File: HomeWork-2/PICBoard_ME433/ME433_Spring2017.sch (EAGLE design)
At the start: 13 parts, among them J6 USB_MINI-B_SMT, Q1 MCP1702

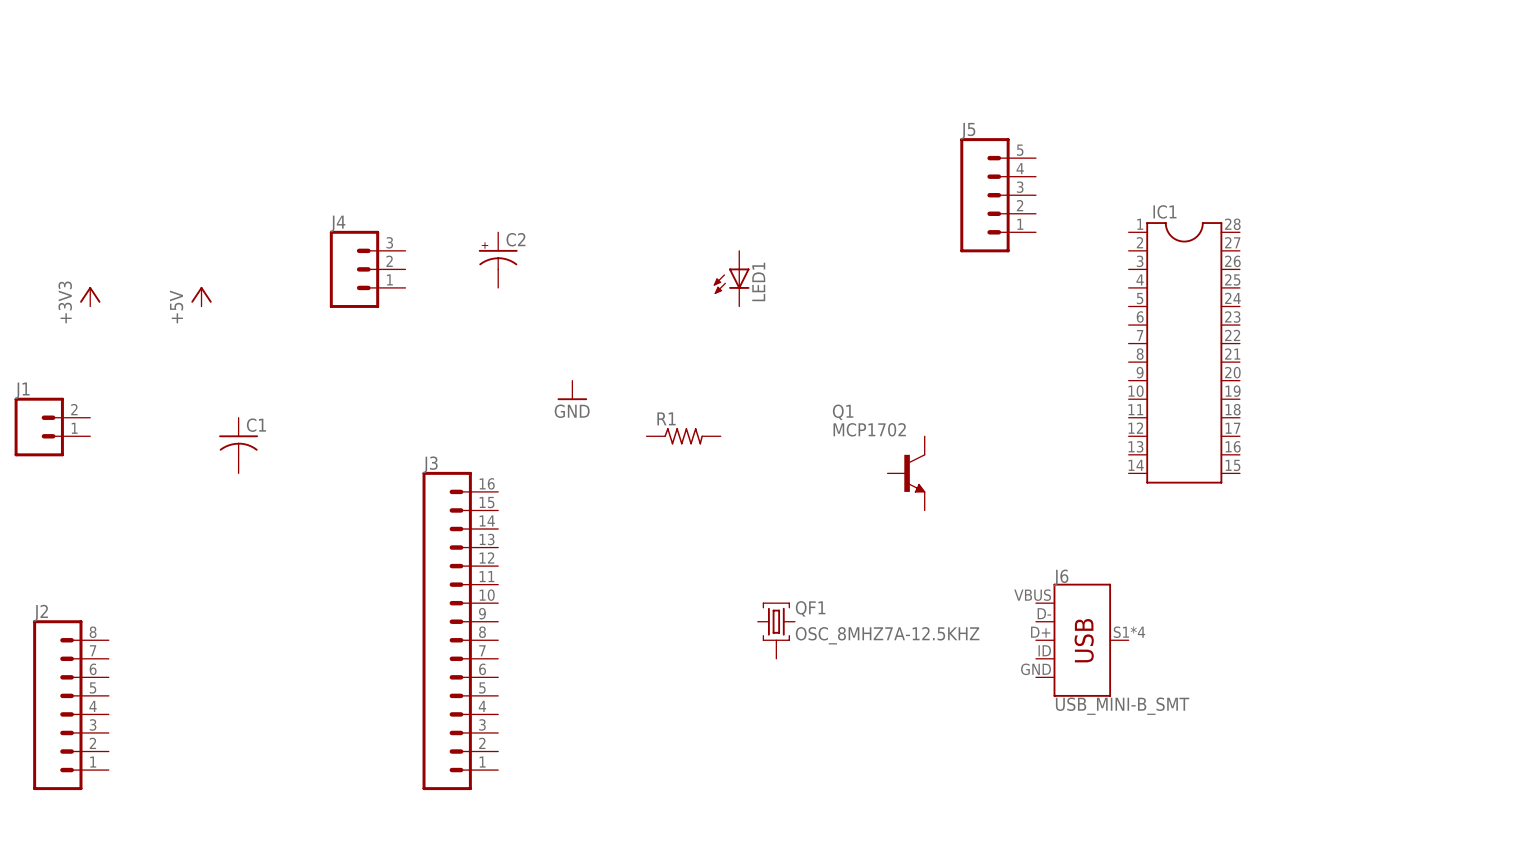
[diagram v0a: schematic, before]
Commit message: Schematic Version #1
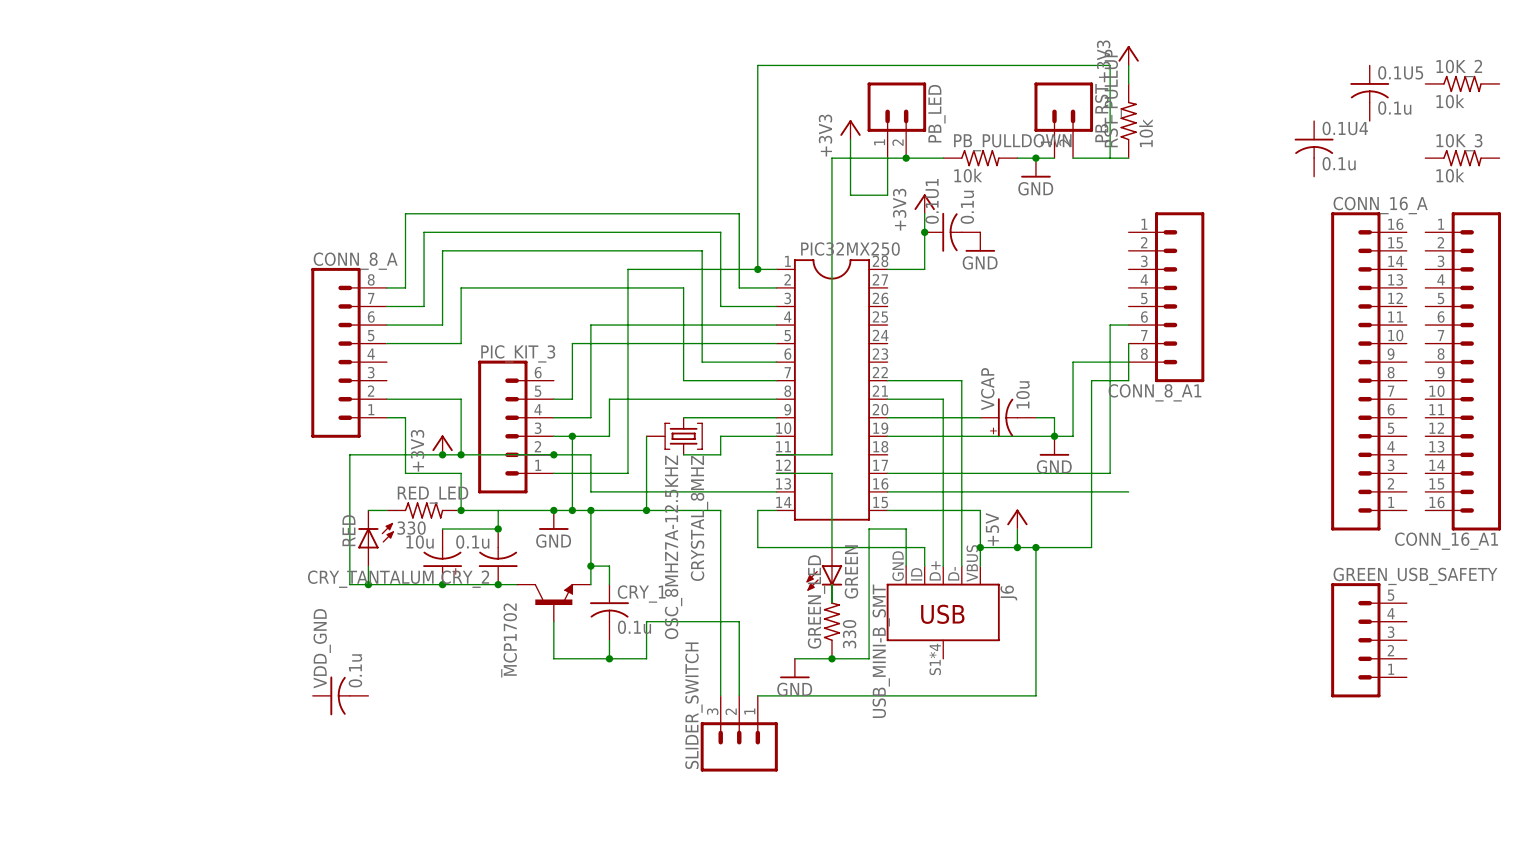
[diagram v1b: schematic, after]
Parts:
- removed C1: (no value), ME433_Spring2017:C-US025-025X050
- removed C2: (no value), ME433_Spring2017:CPOL-USB45181B
- removed IC1: (no value), ME433_Spring2017:PIC-3
- removed J1: (no value), ME433_Spring2017:BUTTONS
- removed J2: (no value), ME433_Spring2017:CONN_08"
- removed J3: (no value), ME433_Spring2017:CONN_16
- removed J4: (no value), ME433_Spring2017:SLIDER_SWITCH
- removed J5: (no value), ME433_Spring2017:USB_GREENBOARD_PULLOUT
- removed LED1: (no value), ME433_Spring2017:LEDSFH482
- removed Q1: MCP1702, ME433_Spring2017:MCP1702
- removed QF1: OSC_8MHZ7A-12.5KHZ, ME433_Spring2017:OSC_8MHZ7A-12.5KHZ
- removed R1: (no value), ME433_Spring2017:R-US_0204/7
- added 0.1U1, 0.1U4, 0.1U5, CRY_1, CRY_2, VDD_GND: 0.1u, ME433_Spring2017:C-US025-025X050
- added 10K_2, 10K_3, PB_PULLDOWN, RST_PULLUP: 10k, ME433_Spring2017:R-US_0204/7
- added CONN_16_A, CONN_16_A1: (no value), ME433_Spring2017:CONN_16
- added CONN_8_A, CONN_8_A1: (no value), ME433_Spring2017:CONN_08"
- added CRYSTAL_8MHZ: OSC_8MHZ7A-12.5KHZ, ME433_Spring2017:OSC_8MHZ7A-12.5KHZ
- added CRY_TANTALUM, VCAP: 10u, ME433_Spring2017:CPOL-USB45181B
- added GREEN, RED: (no value), ME433_Spring2017:LEDSFH482
- added GREEN_LED, RED_LED: 330, ME433_Spring2017:R-US_0204/7
- added GREEN_USB_SAFETY: (no value), ME433_Spring2017:USB_GREENBOARD_PULLOUT
- added PB_LED, PB_RST: (no value), ME433_Spring2017:BUTTONS
- added PIC32MX250: (no value), ME433_Spring2017:PIC-3
- added PIC_KIT_3: (no value), ME433_Spring2017:PICKIT3NO_SILK_FEMALE_PTH
- added SLIDER_SWITCH: (no value), ME433_Spring2017:SLIDER_SWITCH
- added _: MCP1702, ME433_Spring2017:MCP1702
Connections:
- new net +3V3: 0.1U1.1, CONN_8_A.2, CRY_2.1, CRY_TANTALUM.+, PB_LED.1, PIC32MX250.13, PIC32MX250.28, PIC_KIT_3.2, RED.A, RST_PULLUP.2, _.C
- new net +5V: CONN_8_A1.7, J6.VBUS, PIC32MX250.15, SLIDER_SWITCH.1
- new net GND: 0.1U1.2, CONN_8_A.1, CONN_8_A1.8, CRYSTAL_8MHZ.2, CRY_1.1, CRY_2.2, CRY_TANTALUM.-, GREEN_LED.1, J6.GND, PB_PULLDOWN.2, PB_RST.1, PIC32MX250.19, PIC32MX250.8, PIC_KIT_3.3, RED_LED.2, SLIDER_SWITCH.3, VCAP.-, _.E
- new net N$1: CONN_8_A.8, PIC32MX250.2
- new net N$10: PB_LED.2, PB_PULLDOWN.1, PIC32MX250.11
- new net N$11: PIC32MX250.20, VCAP.+
- new net N$12: J6.D+, PIC32MX250.21
- new net N$13: J6.D-, PIC32MX250.22
- new net N$14: CRY_1.2, SLIDER_SWITCH.2, _.B
- new net N$15: PB_RST.2, PIC32MX250.1, PIC_KIT_3.1, RST_PULLUP.1
- new net N$16: RED.C, RED_LED.1
- new net N$17: CONN_8_A.7, PIC32MX250.3
- new net N$18: CONN_8_A.5, PIC32MX250.7
- new net N$2: PIC32MX250.4, PIC_KIT_3.4
- new net N$22: PIC32MX250.16
- new net N$23: CONN_8_A1.6, PIC32MX250.17
- new net N$3: PIC32MX250.5, PIC_KIT_3.5
- new net N$4: GREEN.A, PIC32MX250.12
- new net N$5: CRYSTAL_8MHZ.1, PIC32MX250.9
- new net N$6: CRYSTAL_8MHZ.3, PIC32MX250.10
- new net N$7: GREEN.C, GREEN_LED.2
- new net N$8: J6.ID, PIC32MX250.14
- new net N$9: CONN_8_A.6, PIC32MX250.6
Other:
- moved on the sheet: J6

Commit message: Schematic Version #2
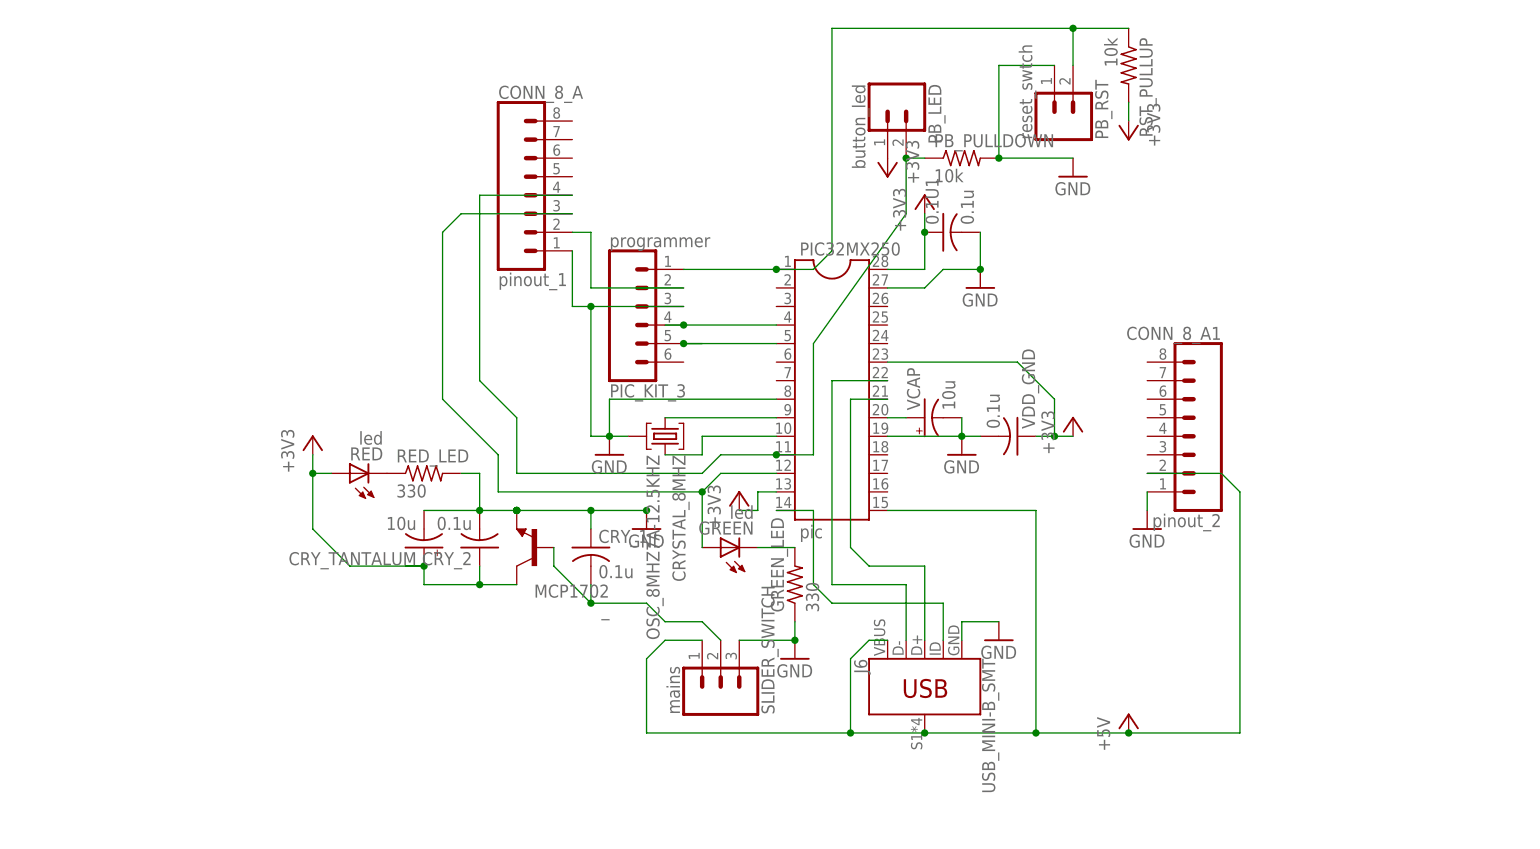
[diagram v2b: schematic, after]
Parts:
- removed 0.1U4, 0.1U5: 0.1u, ME433_Spring2017:C-US025-025X050
- removed 10K_2, 10K_3: 10k, ME433_Spring2017:R-US_0204/7
- removed CONN_16_A, CONN_16_A1: (no value), ME433_Spring2017:CONN_16
- removed GREEN_USB_SAFETY: (no value), ME433_Spring2017:USB_GREENBOARD_PULLOUT
- CONN_8_A: value (none) -> pinout_1
- CONN_8_A1: value (none) -> pinout_2
- GREEN, RED: value (none) -> led
- PB_LED: value (none) -> button_led
- PB_RST: value (none) -> reset_swtch
- PIC32MX250: value (none) -> pic
- PIC_KIT_3: value (none) -> programmer
- SLIDER_SWITCH: value (none) -> mains
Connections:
- removed net N$17: CONN_8_A.7, PIC32MX250.3
- removed net N$18 (its old number): CONN_8_A.5, PIC32MX250.7
- removed net N$22: PIC32MX250.16
- removed net N$23: CONN_8_A1.6, PIC32MX250.17
- removed net N$4 (its old number): GREEN.A, PIC32MX250.12
- removed net N$9 (its old number): CONN_8_A.6, PIC32MX250.6
- new net N$3: CONN_8_A.3, GREEN.A, PIC32MX250.12
- net +3V3: now also PIC32MX250.23, VDD_GND.1; no longer CONN_8_A.2, PIC_KIT_3.2
- net +5V: now also CONN_8_A1.2, J6.SHIELD; no longer CONN_8_A1.7
- net GND: now also CONN_8_A1.1, PIC32MX250.27, VDD_GND.2; no longer CONN_8_A1.8
- net N$1: now also CONN_8_A.2, PIC_KIT_3.2; no longer CONN_8_A.8, PIC32MX250.2
- net N$10: now also CONN_8_A.4
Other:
- moved on the sheet: CONN_8_A, CONN_8_A1, CRYSTAL_8MHZ, CRY_1, CRY_2, CRY_TANTALUM, GREEN, GREEN_LED, J6, PB_PULLDOWN, PB_RST, PIC_KIT_3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
